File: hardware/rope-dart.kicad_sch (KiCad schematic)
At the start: 3 parts, among them IC1 MAX4906ELB+T, U1 ESP32-C3-MINI-1, U2 MAX77751FEFG+

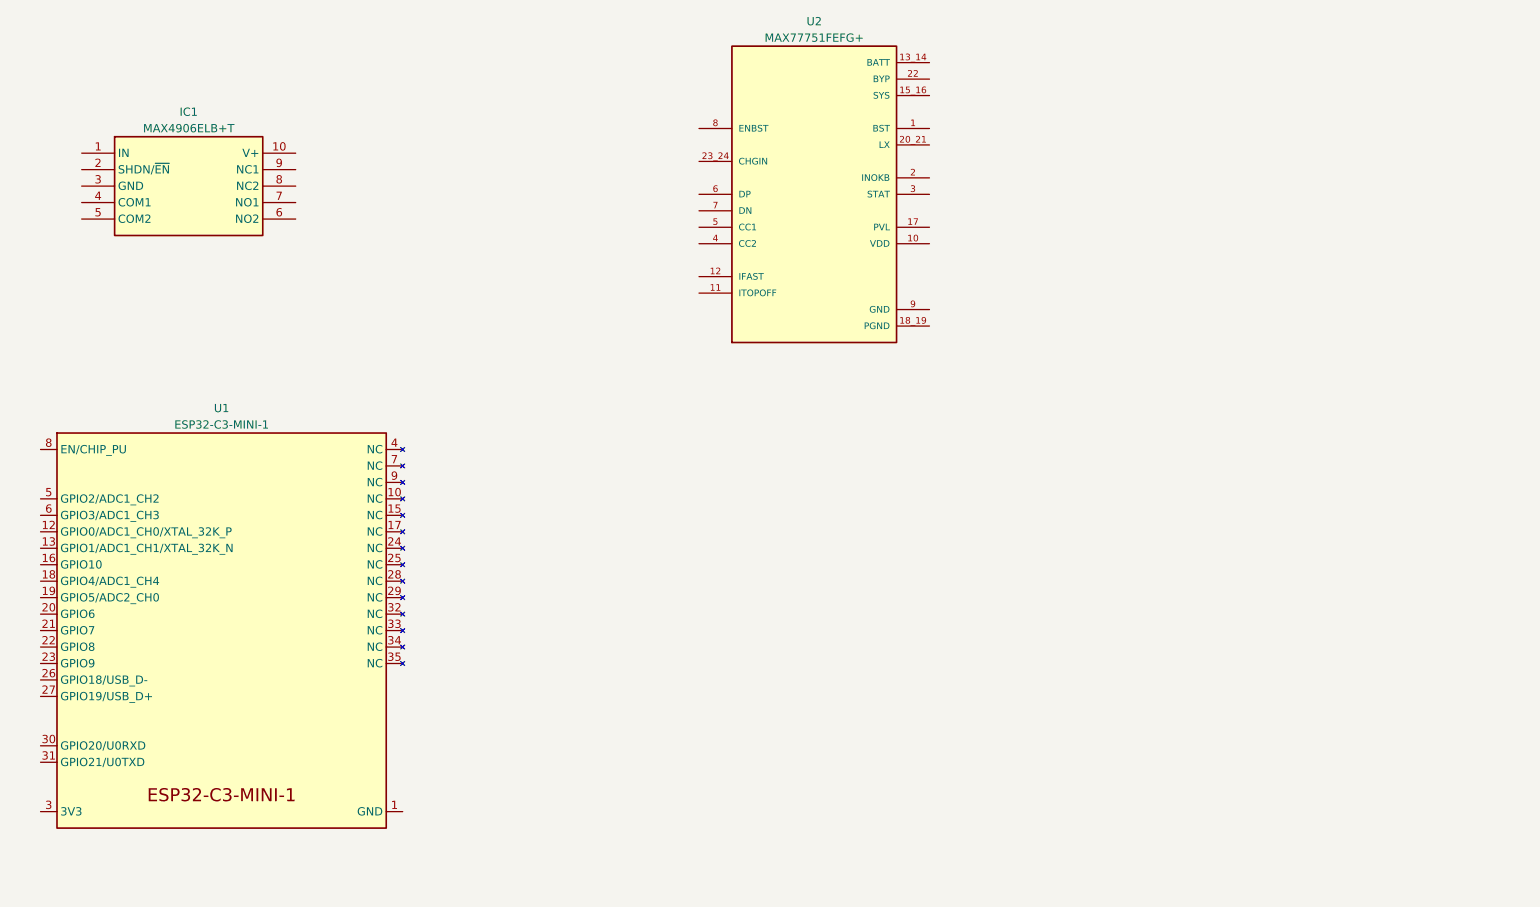
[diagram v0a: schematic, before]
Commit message: started charging shematics
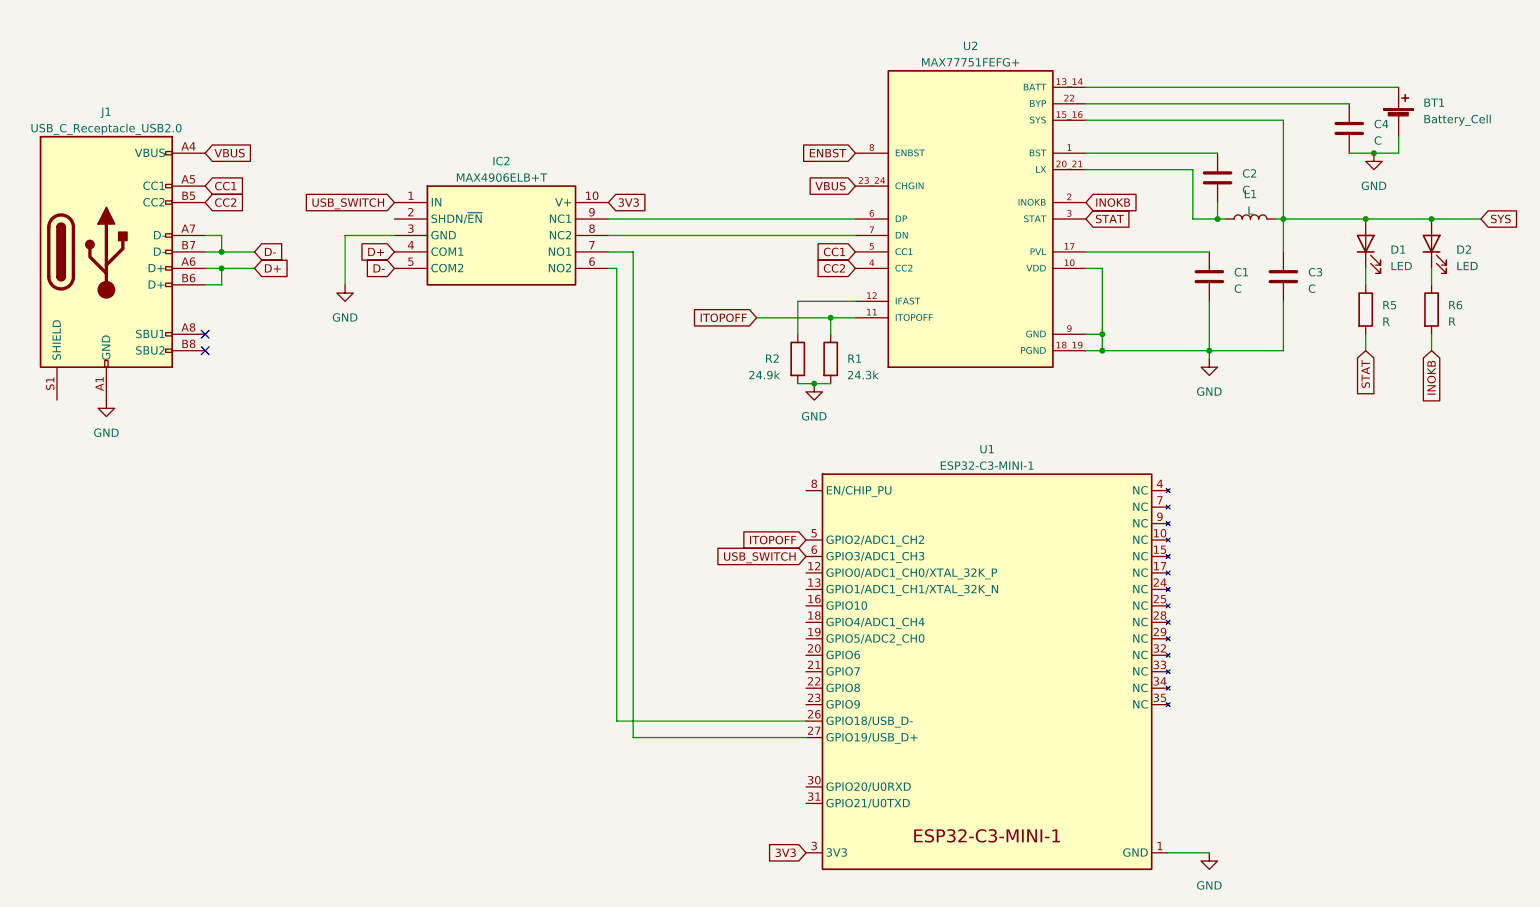
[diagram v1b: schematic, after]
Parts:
- removed IC1: MAX4906ELB+T, MAX4906ELBT, symbol MAX4906ELB+T:MAX4906ELB+T
- added BT1: Battery_Cell, symbol Device:Battery_Cell
- added C1, C2, C3, C4: C, symbol Device:C
- added D1, D2: LED, symbol Device:LED
- added IC2: MAX4906ELB+T, MAX4906ELBT, symbol MAX4906ELB+T:MAX4906ELB+T
- added J1: USB_C_Receptacle_USB2.0, symbol Connector:USB_C_Receptacle_USB2.0
- added L1: L, symbol Device:L
- added R1: 24.3k, symbol Device:R
- added R2: 24.9k, symbol Device:R
- added R5, R6: R, symbol Device:R
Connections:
- net GND: now reaches U1.1 (GND), U1.2 (GND), U1.36 (GND), U1.37 (GND), U1.38 (GND), U1.39 (GND), U1.40 (GND), U1.41 (GND), U1.42 (GND), U1.43 (GND), U1.44 (GND), U1.45 (GND), U1.46 (GND), U1.47 (GND), U1.48 (GND), U1.49 (GND), U1.50 (GND), U1.51 (GND), U1.52 (GND), U1.53 (GND)
- net GND: now also U2.10 (VDD), U2.18_19 (PGND), U2.9 (GND), BT1.2 (-), C1.2, C3.2, C4.2, IC2.3 (GND), J1.A1 (GND), J1.A12 (GND), J1.B1 (GND), J1.B12 (GND), R1.2, R2.2
- net at U1.26 (GPIO18/USB_D-): now also IC2.6 (NO2)
- net at U1.27 (GPIO19/USB_D+): now also IC2.7 (NO1)
- net 3V3: now reaches U1.3 (3V3)
- net 3V3: now also IC2.10 (V+)
- net ITOPOFF: now reaches U1.5 (GPIO2/ADC1_CH2)
- net ITOPOFF: now also U2.11 (ITOPOFF), R1.1
- net USB_SWITCH: now reaches U1.6 (GPIO3/ADC1_CH3)
- net USB_SWITCH: now also IC2.1 (IN)
- net at U2.1 (BST): now also C2.1
- net at U2.12 (IFAST): now also R2.1
- net at U2.13_14 (BATT): now also BT1.1 (+)
- net SYS: now reaches U2.15_16 (SYS)
- net SYS: now also C3.1, D1.2 (A), D2.2 (A), L1.2
- net at U2.17 (PVL): now also C1.1
- net INOKB: now reaches U2.2 (INOKB)
- net INOKB: now also R6.2
- net at U2.20_21 (LX): now also C2.2, L1.1
- net at U2.22 (BYP): now also C4.1
- net VBUS: now reaches U2.23_24 (CHGIN)
- net VBUS: now also J1.A4 (VBUS), J1.A9 (VBUS), J1.B4 (VBUS), J1.B9 (VBUS)
- net STAT: now reaches U2.3 (STAT)
- net STAT: now also R5.2
- net CC2: now reaches U2.4 (CC2)
- net CC2: now also J1.B5 (CC2)
- net CC1: now reaches U2.5 (CC1)
- net CC1: now also J1.A5 (CC1)
- net at U2.6 (DP): now also IC2.9 (NC1)
- net at U2.7 (DN): now also IC2.8 (NC2)
- net ENBST: now reaches U2.8 (ENBST)
- new net: D1.1 (K), R5.1
- new net: D2.1 (K), R6.1
- new net D+: IC2.4 (COM1), J1.A6 (D+), J1.B6 (D+)
- new net D-: IC2.5 (COM2), J1.A7 (D-), J1.B7 (D-)
- no-connect marks 0 -> 2
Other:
- moved on the sheet: U1, U2
